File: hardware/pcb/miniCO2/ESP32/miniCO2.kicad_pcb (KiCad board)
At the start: 4 copper layers, 13.6 x 19.4 mm, 25 parts, among them P1 USB_C_Plug_USB2.0, SW1 SW_Push, SW2 SW_Push, U1 ESP32-C6-MINI-1/U, U2 LM3281, U3 SCD40-D-R2, U4 SIT1552AI-JE-DCC-32.768D

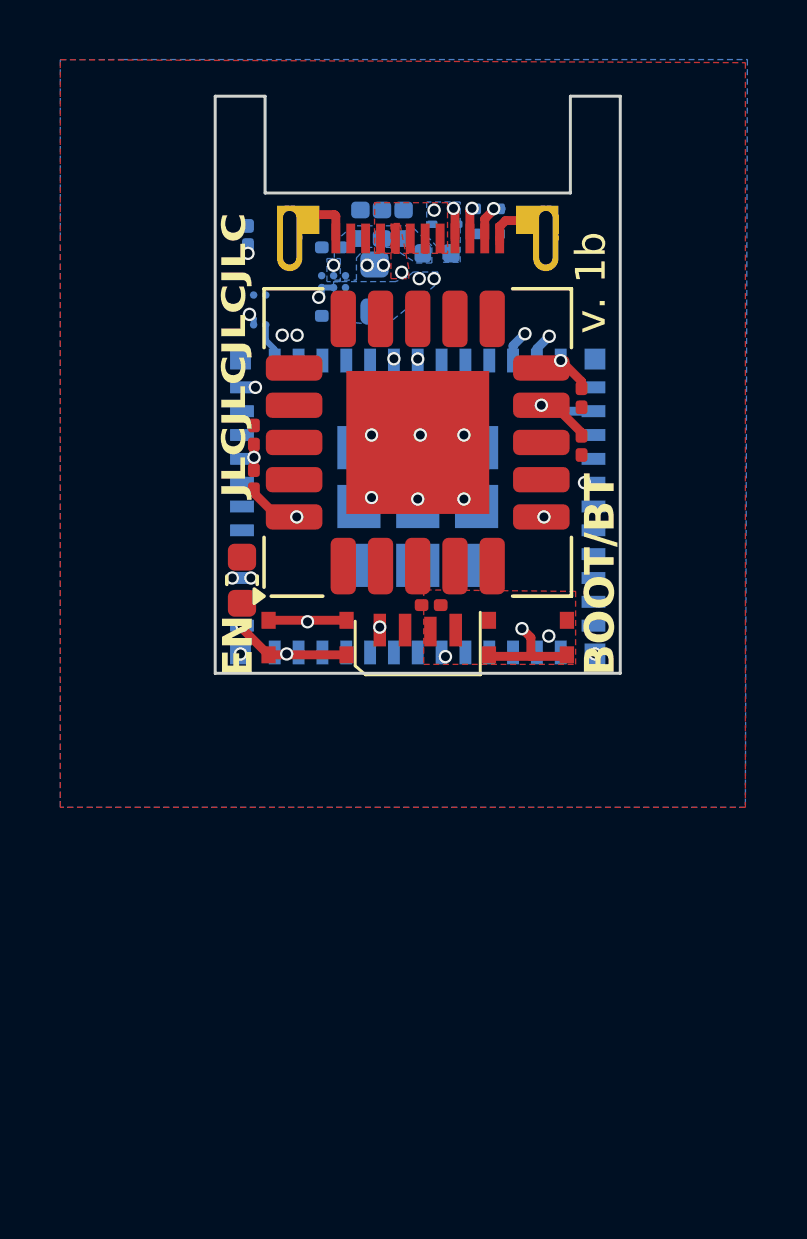
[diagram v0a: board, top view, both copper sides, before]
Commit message: First commit of version 2
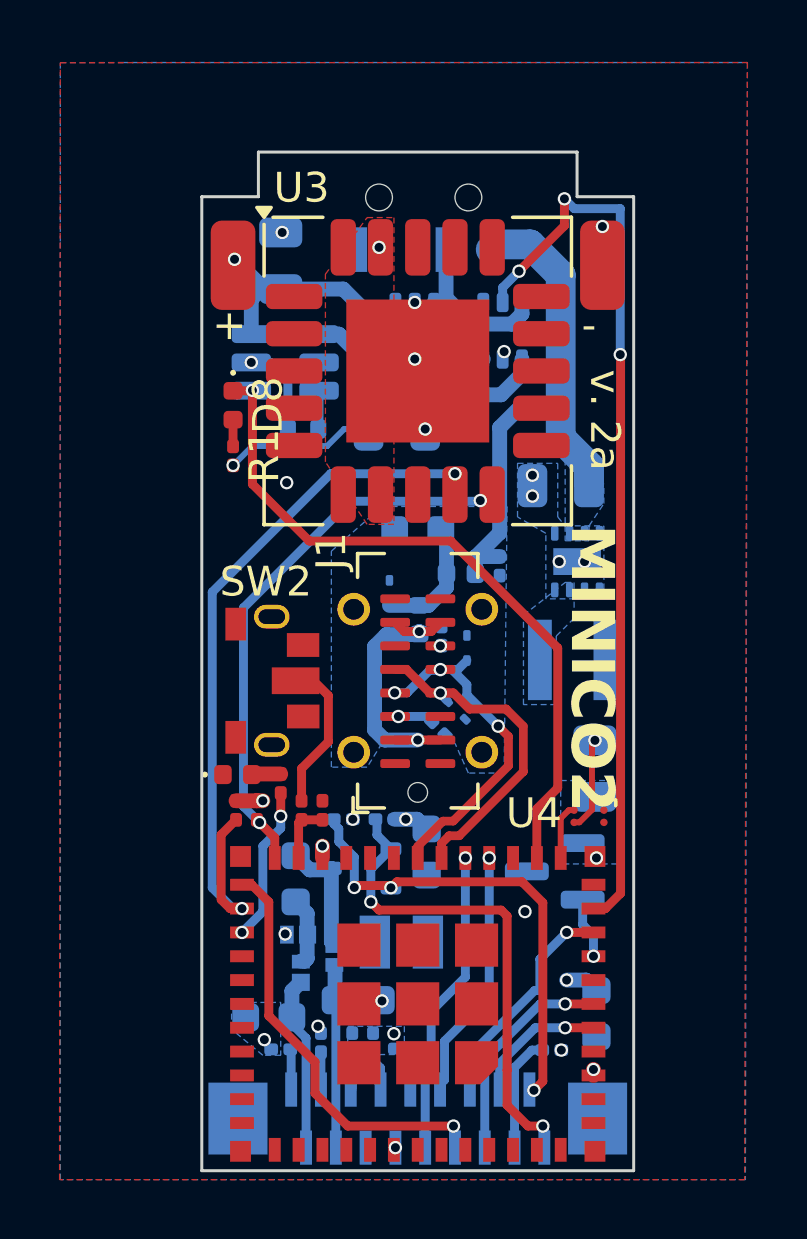
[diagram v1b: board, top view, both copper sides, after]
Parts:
- removed P1: USB_C_Plug_USB2.0, miniCO2:U261-121N-4BS2S
- removed SW1: SW_Push, miniCO2:LS75C2D-T
- added C10: 100n, Capacitor_SMD:C_0201_0603Metric, B.Cu at (144.2, 94.7)
- added C11: 2.2uF, Capacitor_SMD:C_0201_0603Metric, B.Cu at (139.2, 110.7)
- added C12: 2.2uF, Capacitor_SMD:C_0201_0603Metric, B.Cu at (138.2, 110.7)
- added C13: 2.2uF, Capacitor_SMD:C_0201_0603Metric, B.Cu at (136.8, 111.0)
- added C14: 100n, Capacitor_SMD:C_0201_0603Metric, B.Cu at (141.0, 110.9)
- added C15: 4.7uF/25V, Capacitor_SMD:C_0603_1608Metric, B.Cu at (137.3, 105.2)
- added C17: 1uF/25V, Capacitor_SMD:C_0603_1608Metric, B.Cu at (136.4, 109.9)
- added C18: 4.7uF/25V, Capacitor_SMD:C_0603_1608Metric, B.Cu at (141.7, 104.3)
- added C19: 22uF, Capacitor_SMD:C_0805_2012Metric, B.Cu at (136.8, 84.5)
- added C9: 10n, Capacitor_SMD:C_0603_1608Metric, B.Cu at (141.4, 93.5)
- added D5: CUS10S30,H3F, Diode_SMD:D_SOD-323, B.Cu at (144.0, 89.4)
- added D6: NSR05F30NXT5G, miniCO2:XDFN-2(0.6x1), B.Cu at (137.4, 107.1)
- added D7: NSR05F30NXT5G, miniCO2:XDFN-2(0.6x1), B.Cu at (138.6, 107.7)
- added D8: LED_orange, LED_SMD:LED_0402_1005Metric, F.Cu at (135.2, 89.3)
- added D9: LED_green, LED_SMD:LED_0402_1005Metric, F.Cu at (135.4, 101.7)
- added FB1: BLM15PX471SN1D, Inductor_SMD:L_0402_1005Metric, B.Cu at (142.9, 95.0)
- added H1: MountingHole_Pad, Connector_Wire:SolderWirePad_1x01_SMD_1x2mm, F.Cu at (135.2, 84.6)
- added H2: MountingHole_Pad, Connector_Wire:SolderWirePad_1x01_SMD_1x2mm, F.Cu at (147.6, 84.6)
- added J1: USB_C_16P, miniCO2:USB_C_Receptacle_G-Switch_GT-USB-7051x, F.Cu at (141.4, 98.6)
- added J2: Conn_01x18, miniCO2:XKB Connection X05C2018TZ, B.Cu at (141.4, 113.3)
- added L2: 47u, miniCO2:L_SMD_2.2x1.6mm, B.Cu at (140.9, 107.4)
- added Q2: Si1308EDL, Package_TO_SOT_SMD:SOT-323_SC-70, B.Cu at (139.5, 104.9)
- added R10: 5.1k, Resistor_SMD:R_0201_0603Metric, F.Cu at (136.8, 102.0)
- added R2: 5.1k, Resistor_SMD:R_0201_0603Metric, B.Cu at (142.2, 97.1)
- added R3: 5.1k, Resistor_SMD:R_0201_0603Metric, B.Cu at (142.1, 100.2)
- added R5: 2.2, Resistor_SMD:R_0201_0603Metric, B.Cu at (138.9, 103.2)
- added R8: 5.6k, Resistor_SMD:R_0402_1005Metric, B.Cu at (137.6, 90.1)
- added R9: 5.1k, Resistor_SMD:R_0201_0603Metric, F.Cu at (137.5, 102.9)
- added SW3: MK-12C03-G015, miniCO2:MK-12C03-G015, B.Cu at (141.6, 82.4)
- added U5: SLM6401, Package_TO_SOT_SMD:SOT-23-6, B.Cu at (137.0, 87.9)
- added U6: LM66100DCK, Package_TO_SOT_SMD:SOT-363_SC-70-6, B.Cu at (141.3, 86.8)
- added U7: LM66100DCK, Package_TO_SOT_SMD:SOT-363_SC-70-6, B.Cu at (144.3, 86.8)
- added U8: TPS62172DSG, Package_SON:WSON-8-1EP_2x2mm_P0.5mm_EP0.9x1.6mm, B.Cu at (146.8, 94.6)
- C1, C3: value 2.2uF -> 22uF; footprint Capacitor_SMD:C_0201_0603Metric -> Capacitor_SMD:C_0805_2012Metric
- C2: value 2.2uF -> 22uF; footprint Capacitor_SMD:C_0201_0603Metric -> Capacitor_SMD:C_0805_2012Metric; moved to B.Cu
- C4: value 10uF -> 4.7uF/25V; moved to B.Cu
- C5: value 22uF -> 2.2uF; footprint Capacitor_SMD:C_0402_1005Metric -> Capacitor_SMD:C_0201_0603Metric
- C6: value 22uF -> 1uF/25V; footprint Capacitor_SMD:C_0402_1005Metric -> Capacitor_SMD:C_0603_1608Metric
- C7: value 100nF -> 2.2uF; moved to B.Cu
- C8: value 22uF -> 100n; footprint Capacitor_SMD:C_0402_1005Metric -> Capacitor_SMD:C_0201_0603Metric; moved to F.Cu
- D1: value WS2812C-4020 -> NSR05F30NXT5G; footprint miniCO2:WS2812C-4020 -> miniCO2:XDFN-2(0.6x1); moved to B.Cu
- F1: value BSMD0402L-075 -> 6V 750mA 40A 1.5A
- L1: value 0.47uH -> 3.3uH; footprint Inductor_SMD:L_0603_1608Metric -> miniCO2:L_Murata_LQH3NPZ
- R4: value 5.1k -> 1M
- SW2: footprint miniCO2:LS75C2D-T -> miniCO2:GT-TC108X-H034
- U1, U4: moved to F.Cu
- U2: value LM3281 -> MAX809TEUR; footprint Package_BGA:Texas_DSBGA-6_0.95x1.488mm_Layout2x3_P0.4mm -> Package_TO_SOT_SMD:SOT-23
- moved C5 28.2 mm to (145.9, 111.0), turned to 180 degrees
- moved C6 26.1 mm to (139.4, 109.3), turned to 180 degrees
- moved U2 21.1 mm to (146.0, 105.0), turned to 180 degrees
- moved U4 20.3 mm to (147.2, 103.1), turned to -90 degrees
- moved R4 20.1 mm to (140.3, 103.2), turned to 0 degrees
- moved C8 19.7 mm to (138.2, 102.9), turned to 90 degrees
- moved C4 18.8 mm to (147.4, 109.8), turned to -90 degrees
- moved R6 17.6 mm to (136.0, 102.9), turned to 90 degrees
- moved C1 17.6 mm to (147.4, 101.5), turned to 90 degrees
- moved R7 16.9 mm to (135.3, 102.9), turned to 90 degrees
- moved U1 16.7 mm to (141.4, 112.1), turned to 180 degrees
- moved D3 16.4 mm to (142.7, 99.6), turned to 135 degrees
- moved C7 14.8 mm to (139.9, 110.7), turned to -90 degrees
- moved D2 14.4 mm to (143.1, 97.5), turned to -90 degrees
- moved L1 14.1 mm to (146.6, 97.9), turned to 0 degrees
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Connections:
- C2 pad 2: EN -> Net-(SW3-C)
- C3 pad 2: Net-(U2-VIN) -> VBUS
- C5 pad 2: Net-(U2-VIN) -> VSHR
- C6 pad 2: Net-(U2-VIN) -> VGH
- C7 pad 1: +3.3V -> GND
- C7 pad 2: GND -> VDD
- C8 pad 1: GND -> BOOT_MODE
- C8 pad 2: Net-(U2-VIN) -> GND
- D1 pad 1: DIN -> Net-(D1-K)
- D1 pad 2: +3.3V -> VGL
- D2 pad 2: D- -> D+
- D3 pad 2: D+ -> D-
- D4 pad 2: VBUS -> Net-(D4-A2)
- F1 pad 1: VBUS -> Net-(F1-Pad1)
- F1 pad 2: Net-(U2-VIN) -> Net-(D4-A2)
- L1 pad 1: Net-(U2-SW) -> Net-(U8-SW)
- R1 pad 1: EN -> Net-(D8-A)
- R1 pad 2: +3.3V -> VBUS
- R4 pad 1: GND -> GDR
- R4 pad 2: Net-(P1-CC) -> GND
- SW2 pad 2: BOOT_MODE -> Net-(R9-Pad2)
- U1 pad 10: unconnected-(U1-MTDI/GPIO5/ADC1_CH5-Pad10) -> VBUS_EN_SENSE
- U1 pad 13: unconnected-(U1-GPIO1/ADC1_CH1/XTAL_32K_N-Pad13) -> CHRG_SENSE
- U1 pad 15: unconnected-(U1-MTCK/GPIO6/ADC1_CH6-Pad15) -> SPISCL
- U1 pad 16: unconnected-(U1-MTDO/GPIO7-Pad16) -> MOSI
- U1 pad 25: unconnected-(U1-GPIO19-Pad25) -> CS#
- U1 pad 27: unconnected-(U1-GPIO21-Pad27) -> Net-(U1-GPIO21)
- U1 pad 29: DIN -> unconnected-(U1-GPIO23-Pad29)
- U1 pad 5: unconnected-(U1-GPIO2/ADC1_CH2-Pad5) -> BUSY
- U1 pad 6: unconnected-(U1-GPIO3/ADC1_CH3-Pad6) -> RES#
- U1 pad 9: unconnected-(U1-MTMS/GPIO4/ADC1_CH4-Pad9) -> D/C#
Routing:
- net VBUS_EN_SENSE: track 0.00 -> 30.5 mm, vias 0 -> 3
- net CHRG_SENSE: track 0.00 -> 23.7 mm, vias 0 -> 1
- net SCL: track 3.69 -> 24.7 mm, vias 1 -> 2
- net GDR: track 0.00 -> 16.6 mm, vias 0 -> 2
- net SDA: track 1.78 -> 18.4 mm, vias 1 -> 2
- net Net-(P1-CC): track 15.9 -> 0.00 mm, vias 2 -> 0
- net RESE: track 0.00 -> 15.8 mm, vias 0 -> 3
- net CS#: track 0.00 -> 13.8 mm, vias 0 -> 1
- net /Input and power/VBAT: track 0.00 -> 13.1 mm, vias 0 -> 1
- net BOOT_MODE: track 14.9 -> 2.02 mm, vias 2 -> 0
- net DIN: track 12.7 -> 0.00 mm, vias 2 -> 0
- net VBUS: track 6.80 -> 17.5 mm, vias 2 -> 1
- net Net-(SW3-C): track 0.00 -> 10.3 mm
- net MOSI: track 0.00 -> 10.3 mm, vias 0 -> 1
- net Net-(F1-Pad1): track 0.00 -> 9.47 mm, vias 0 -> 2
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- added copper zone on In1.Cu, net GND
- added copper zone on B.Cu, net Net-(SW3-C)
- added copper zone on B.Cu, net Net-(U8-SW)
- removed copper zone on B.Cu, net Net-(U2-SW)
- removed copper zone on In2.Cu, net Net-(U2-SW)
- removed copper zone on B.Cu, net Net-(U2-VIN)
- removed copper zone on B.Cu, net VBUS
- removed copper zone on F.Cu, net VBUS
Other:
- board size 13.6 x 19.4 mm -> 14.5 x 34.2 mm
- board text added: "+"
- board text added: "-"
- board text added: "v. 2a"
- board text removed: "BOOT/BT"
- board text removed: "Case edge"
- board text removed: "EN"
- board text removed: "v. 1b"
